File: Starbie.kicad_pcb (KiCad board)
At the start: 2 copper layers, 120 x 90 mm, 7 parts, among them J1 Conn_01x04_Pin, J2 Conn_01x08_Pin, SW1 SW_Push, SW2 SW_Push, U1 XIAO-ESP32-C3-SMD, U2 DHT11

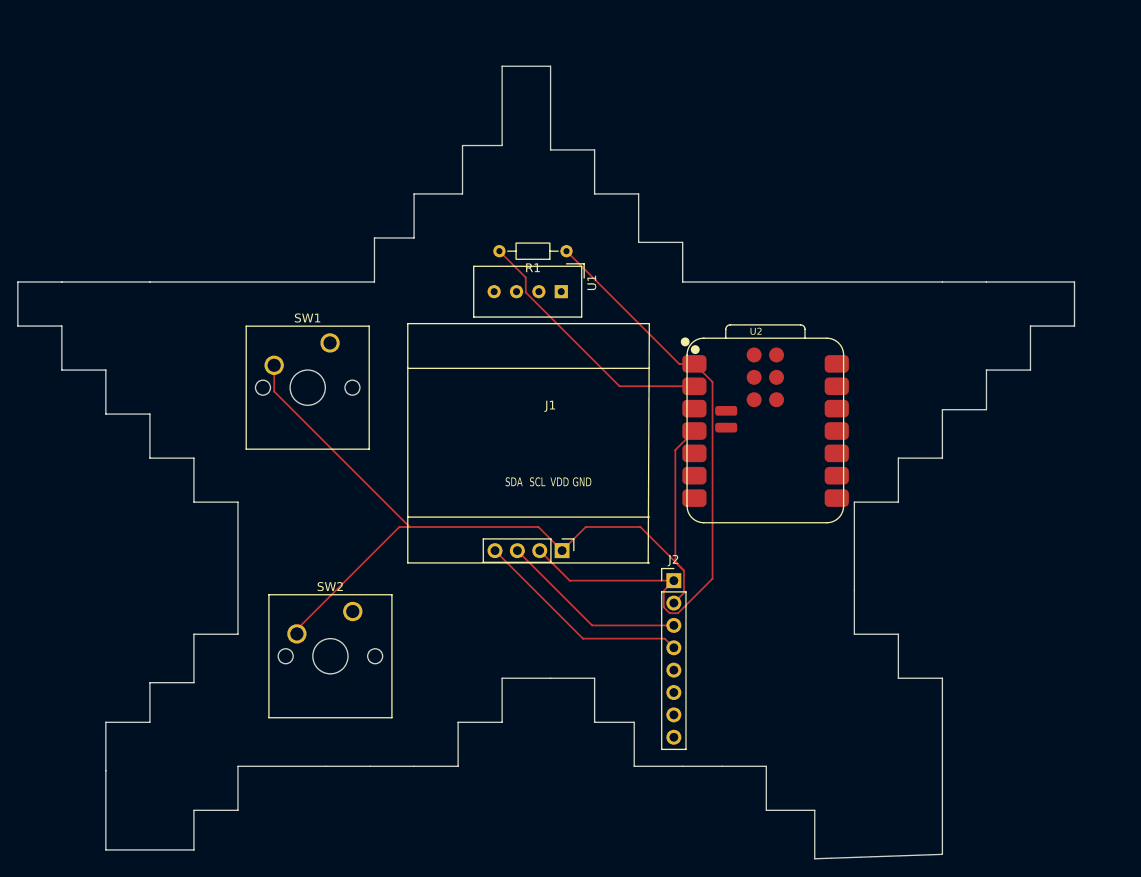
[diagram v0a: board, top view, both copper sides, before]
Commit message: Add files via upload
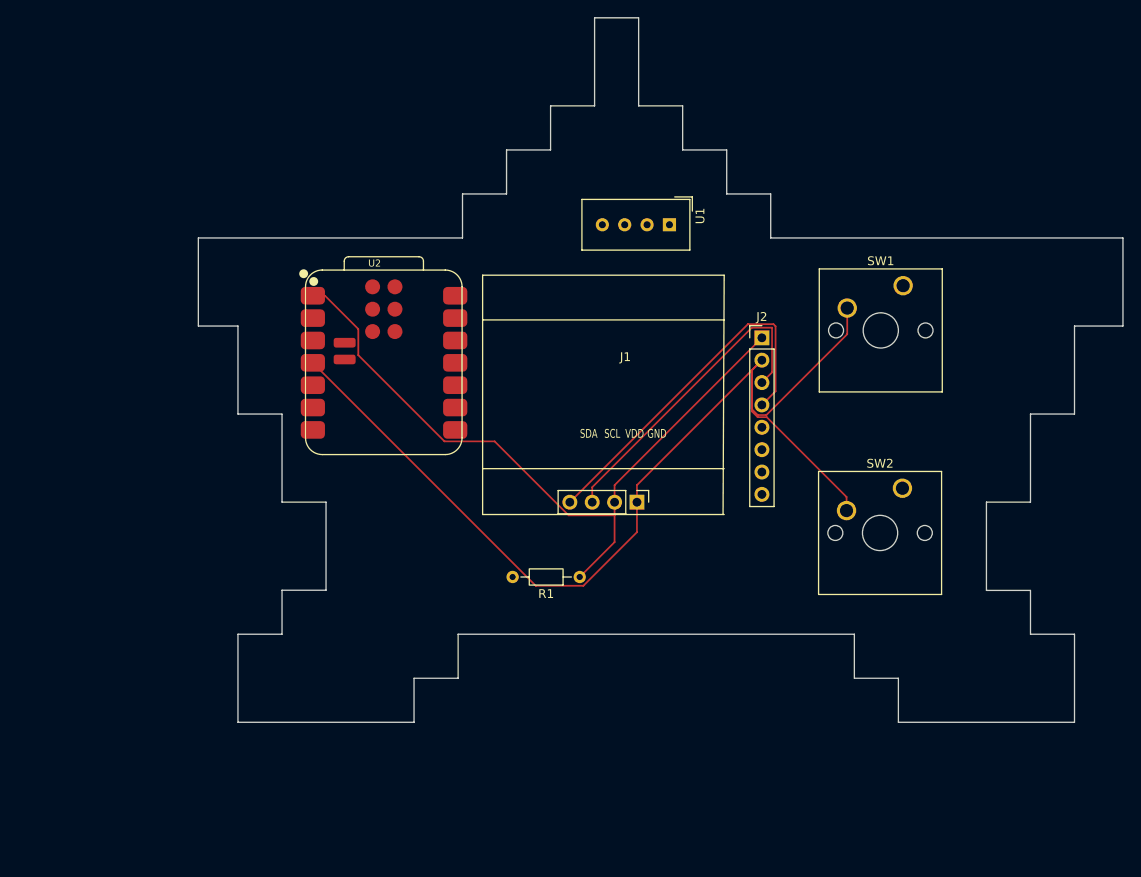
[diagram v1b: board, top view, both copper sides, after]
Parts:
- moved SW1 65.4 mm to (195.5, 70.4)
- moved SW2 64.0 mm to (195.5, 93.4)
- moved U2 44.0 mm to (127.7, 89.7)
- moved R1 37.0 mm to (158.8, 103.5)
- moved J2 29.3 mm to (179.5, 76.3)
- moved U1 14.4 mm to (169.0, 63.5)
- moved J1 10.1 mm to (161.5, 95.0)
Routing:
- net /DHT11 DATA: track 29.5 -> 0.00 mm
- net GND: track 99.7 -> 120.1 mm
- net /SDA: track 24.9 -> 41.4 mm
- net /SCL: track 21.3 -> 36.3 mm
- net +3.3V: track 72.7 -> 82.1 mm
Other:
- board size 120 x 90 mm -> 105 x 80 mm

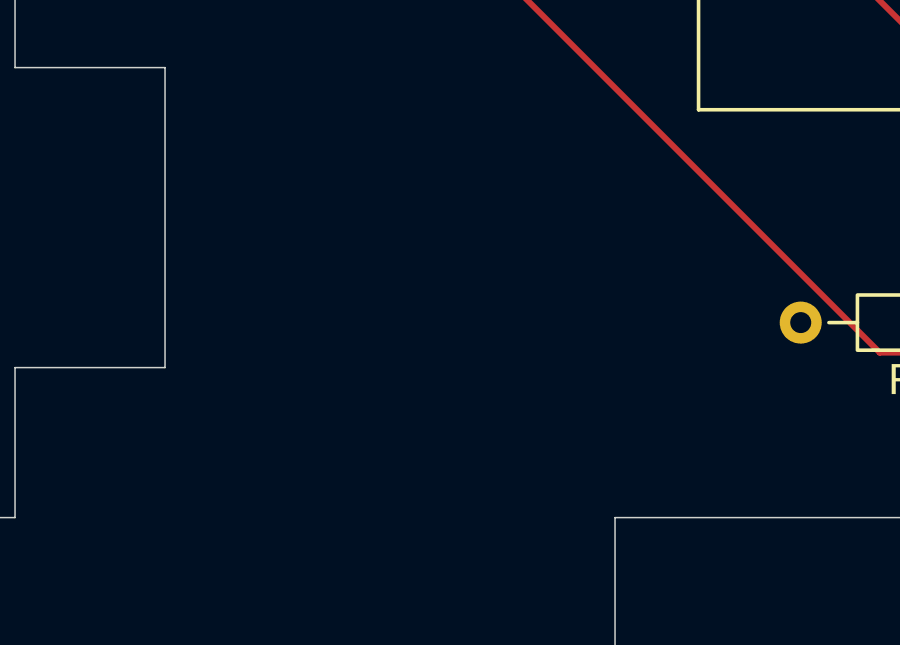
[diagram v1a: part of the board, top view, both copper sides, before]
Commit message: Add files via upload
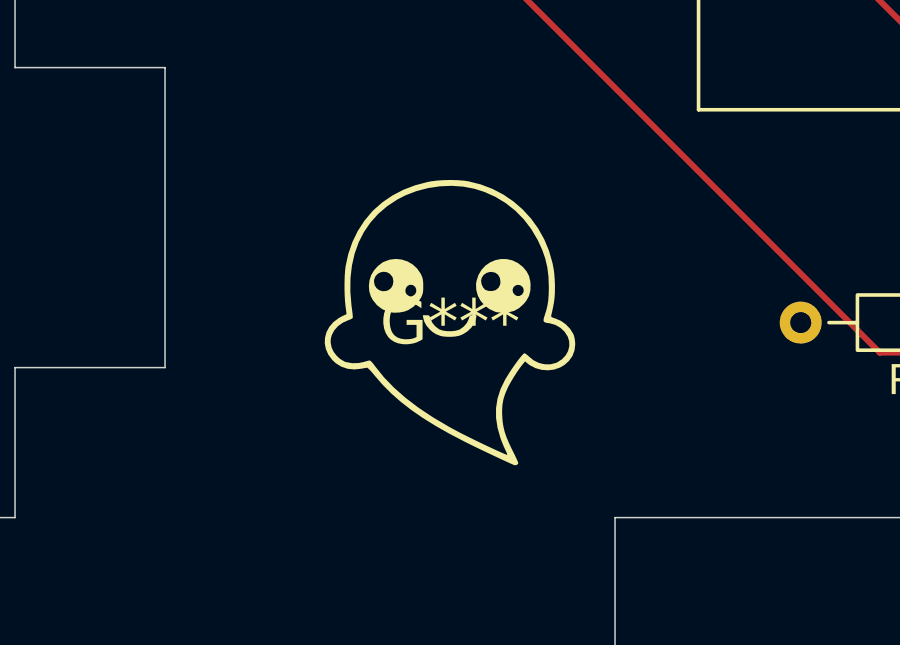
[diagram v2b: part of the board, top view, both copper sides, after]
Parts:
- added G***: LOGO, Ghost:Ghost, F.Cu at (139.5, 103.5)

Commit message: Add files via upload
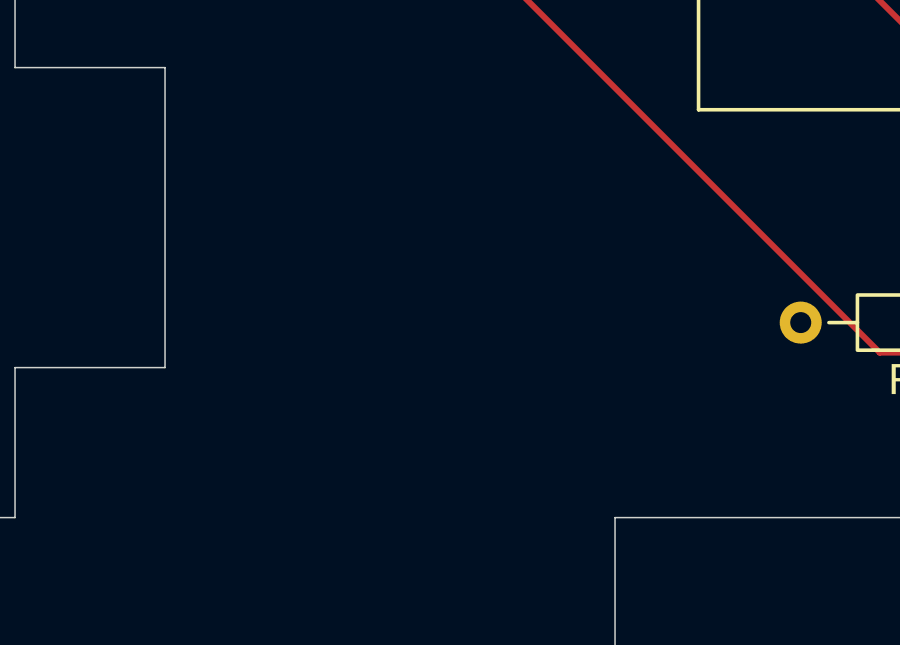
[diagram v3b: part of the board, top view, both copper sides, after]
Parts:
- removed G***: LOGO, Ghost:Ghost
